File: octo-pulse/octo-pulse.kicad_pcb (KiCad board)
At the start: 2 copper layers, 56 x 59 mm, 8 parts, among them SW1 SW_Push, SW2 SW_Push, SW3 SW_Push, SW4 SW_Push, SW5 SW_Push, SW6 SW_Push

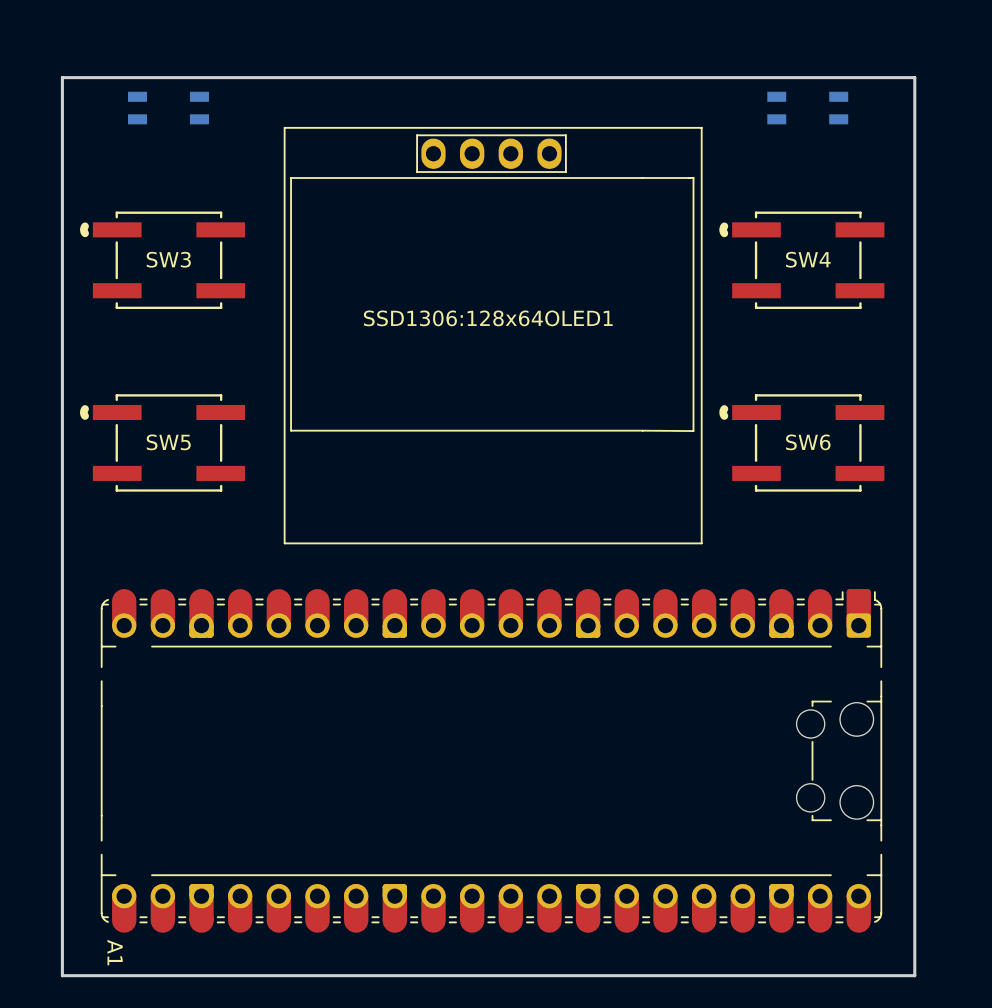
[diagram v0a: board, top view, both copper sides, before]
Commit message: Fully wired PCB in KiCad
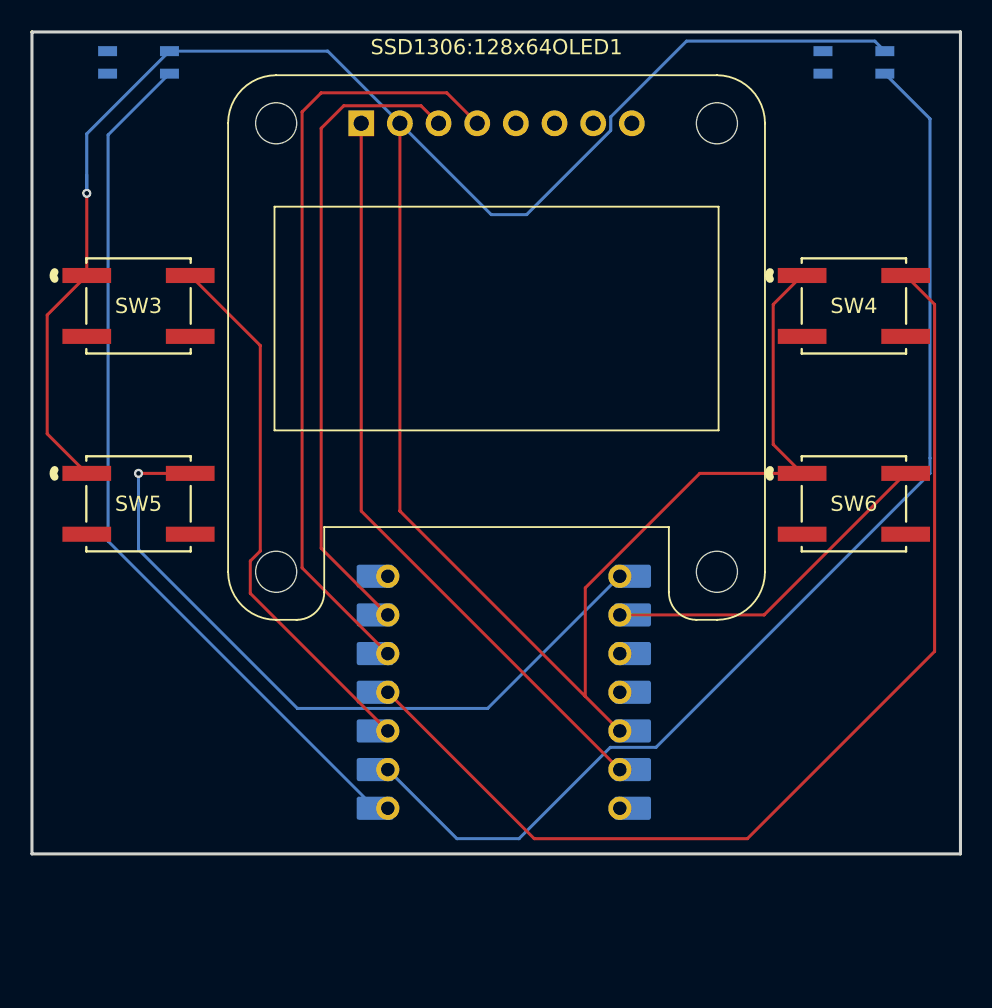
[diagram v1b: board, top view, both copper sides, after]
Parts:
- removed A1: RaspberryPi_Pico, Module:RaspberryPi_Pico_Common_Unspecified
- added U1: XIAO-RP2040-NORMAL, Seeed Studio XIAO Series Library:XIAO-RP2040-DIP, B.Cu at (166.0, 112.4)
- SSD1306:128x64OLED1: footprint SSD1306:128x64OLED -> SSD1306:Adafruit_SSD1306_1.3''
- SW1: value SW_Push -> SW_TL
- SW2: value SW_Push -> SW_TR
- SW3: value SW_Push -> SW_ML
- SW4: value SW_Push -> SW_MR
- SW5: value SW_Push -> SW_BL
- SW6: value SW_Push -> SW_BR
- moved SSD1306:128x64OLED1 15.1 mm to (156.6, 75.0)
- moved SW6 5.00 mm to (189.0, 100.0)
- moved SW5 4.47 mm to (142.0, 100.0)
- moved SW2 4.27 mm to (189.0, 71.0)
- moved SW4 4.24 mm to (189.0, 87.0)
- moved SW3 3.61 mm to (142.0, 87.0)
- moved SW1 3.59 mm to (142.0, 71.0)
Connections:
- SSD1306:128x64OLED1 pad 3: A4 -> SCL
- SSD1306:128x64OLED1 pad 4: A5 -> SDA
- SW1 pad 1: unconnected-(SW1-Pad1) -> VCC
- SW2 pad 1: unconnected-(SW2-Pad1) -> VCC
- SW3 pad 1: unconnected-(SW3-Pad1) -> VCC
- SW4 pad 1: unconnected-(SW4-Pad1) -> VCC
- SW5 pad 1: unconnected-(SW5-Pad1) -> VCC
- SW6 pad 1: unconnected-(SW6-Pad1) -> VCC
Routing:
- net VCC: track 0.00 -> 175.3 mm, vias 0 -> 1
- net Net-(U1-GPIO27/ADC1/A1): track 0.00 -> 74.9 mm
- net Net-(U1-GPIO29/ADC3/A3): track 0.00 -> 70.5 mm
- net Net-(U1-GPIO26/ADC0/A0): track 0.00 -> 58.0 mm
- net SDA: track 0.00 -> 50.8 mm
- net GND: track 0.00 -> 49.5 mm
- net Net-(U1-GPIO1/RX): track 0.00 -> 47.9 mm, vias 0 -> 1
- net SCL: track 0.00 -> 42.6 mm
- net Net-(U1-GPIO28/ADC2/A2): track 0.00 -> 35.8 mm
- net Net-(U1-GPIO2/SCK): track 0.00 -> 22.6 mm
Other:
- board size 56 x 59 mm -> 61 x 54 mm
